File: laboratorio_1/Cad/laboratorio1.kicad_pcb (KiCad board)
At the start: 2 copper layers, 100 x 50 mm, 31 parts, among them J5 Output, U1 TL084, U2 TL084, j1 Vdd, j2 Vss, j3 GND, j4 Input

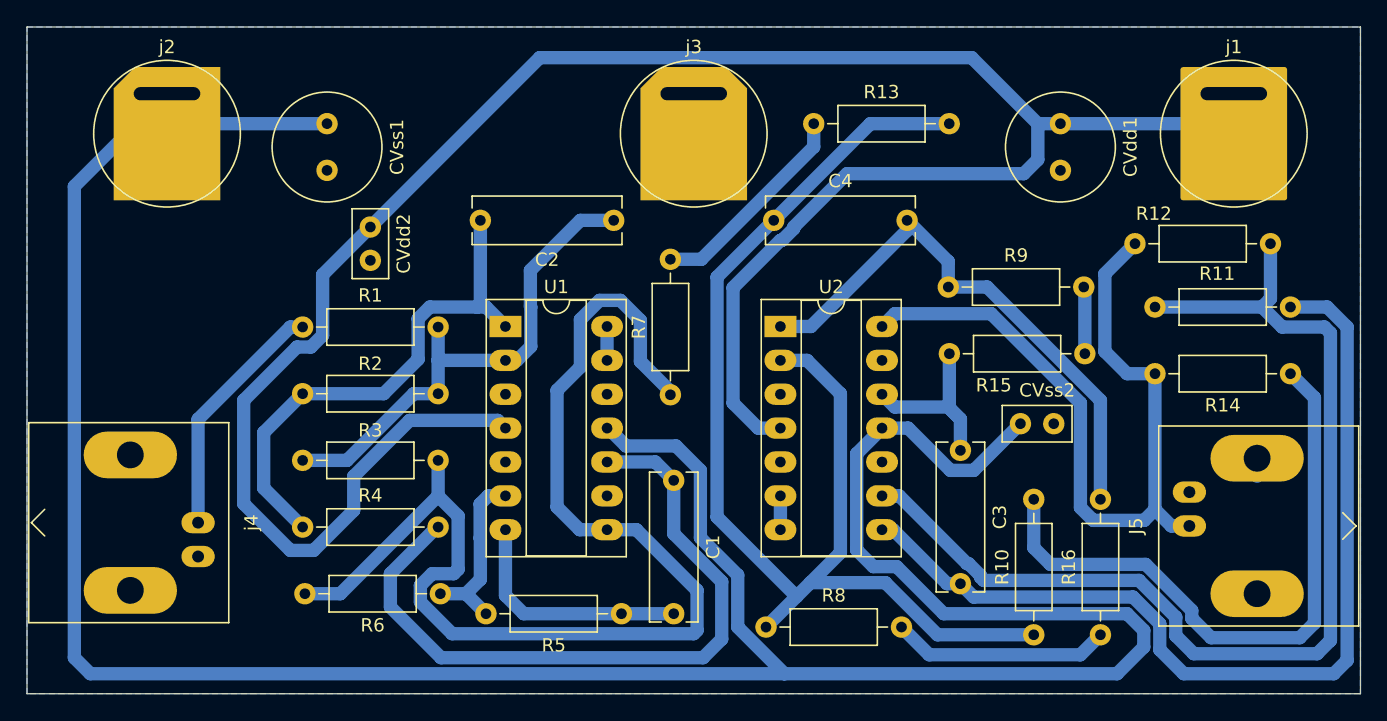
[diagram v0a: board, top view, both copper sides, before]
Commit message: version final
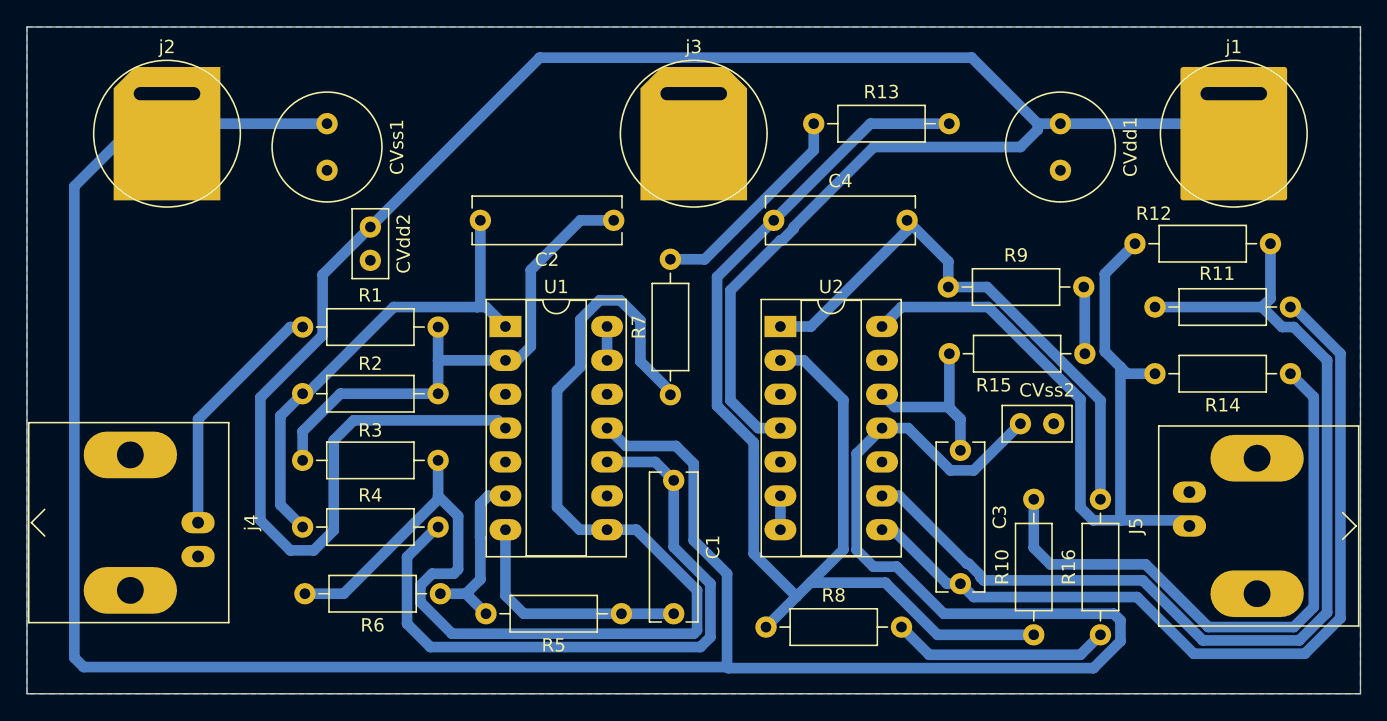
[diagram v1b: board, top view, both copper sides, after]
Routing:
- net Net-(C3-Pad2): track 70.8 -> 64.4 mm
- net Net-(U1E-V-): track 214.2 -> 208.2 mm
- net Net-(U2C--): track 81.9 -> 77.3 mm
- net GND: track 3.60 -> 0.00 mm
- net Net-(U1C-+): track 53.5 -> 50.5 mm
- net Net-(C2-Pad2): track 39.3 -> 36.5 mm
- net Net-(R10-Pad2): track 47.7 -> 45.9 mm
- net Net-(U1A--): track 38.1 -> 39.4 mm
- net Net-(J5-In): track 59.0 -> 60.2 mm
